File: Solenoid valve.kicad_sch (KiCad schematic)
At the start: 21 parts, among them J2 Conn_01x02, J3 Conn_01x02, J4 Conn_01x02, Q1 S8050, Q2 S8050, U1 BTS443P

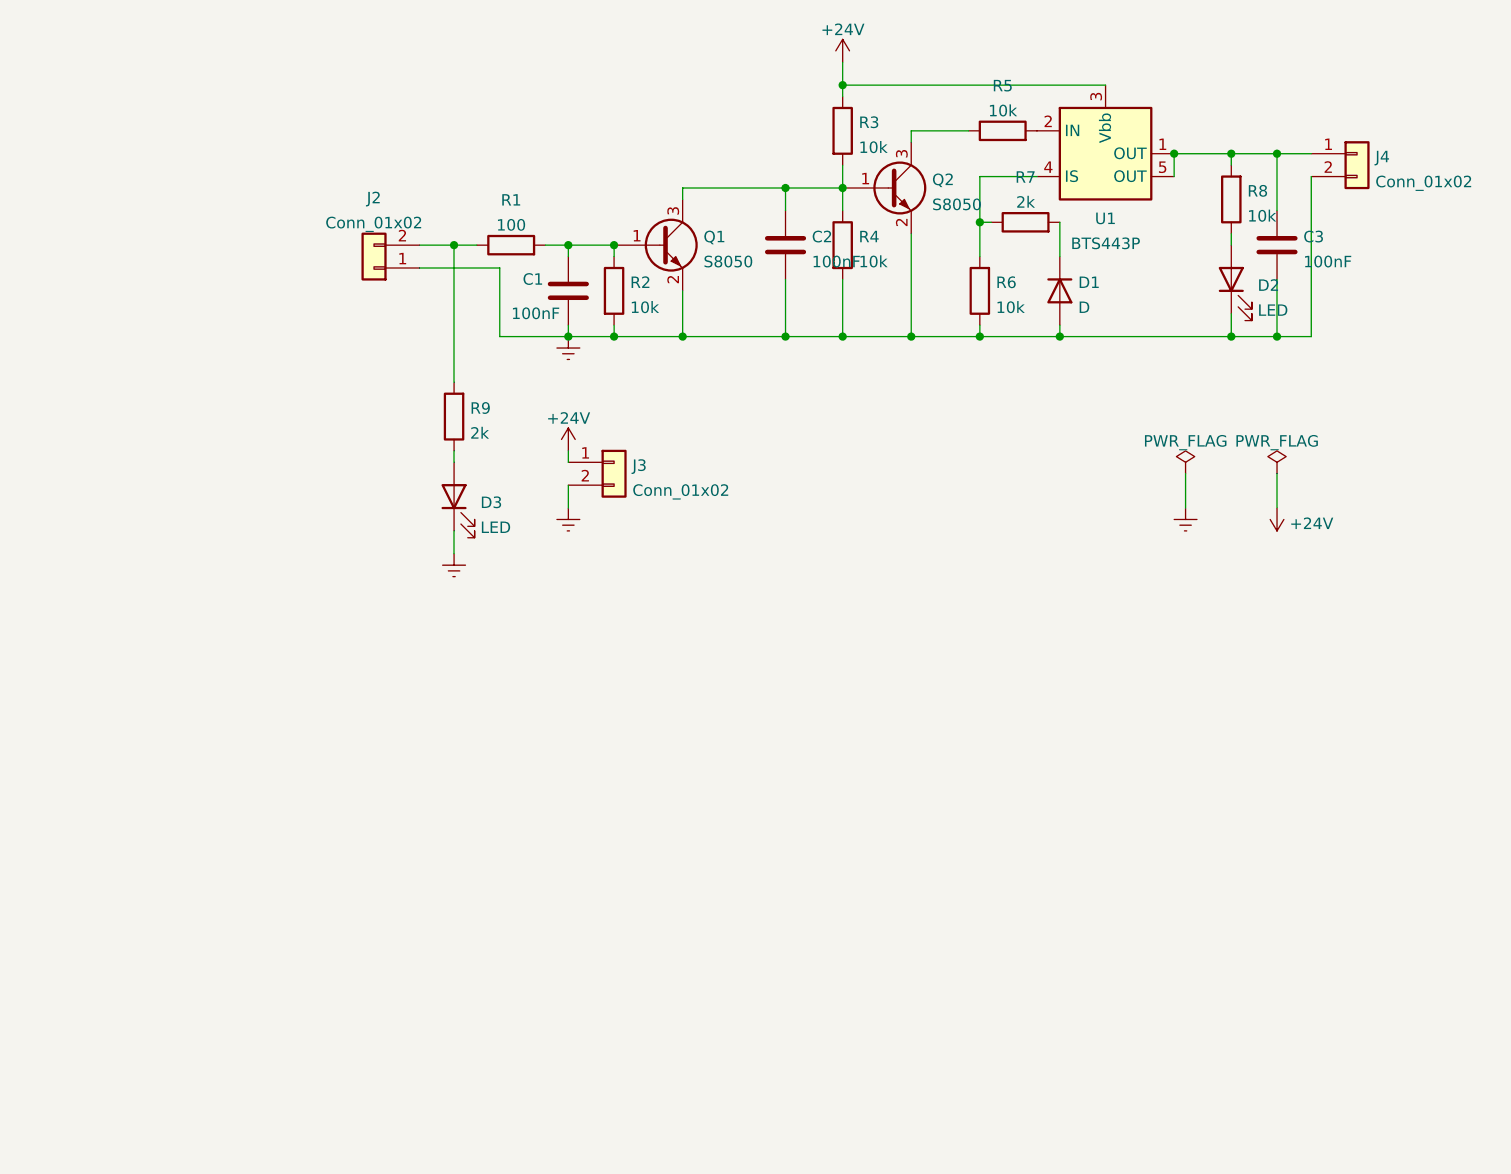
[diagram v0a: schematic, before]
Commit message: Adjustment for full version
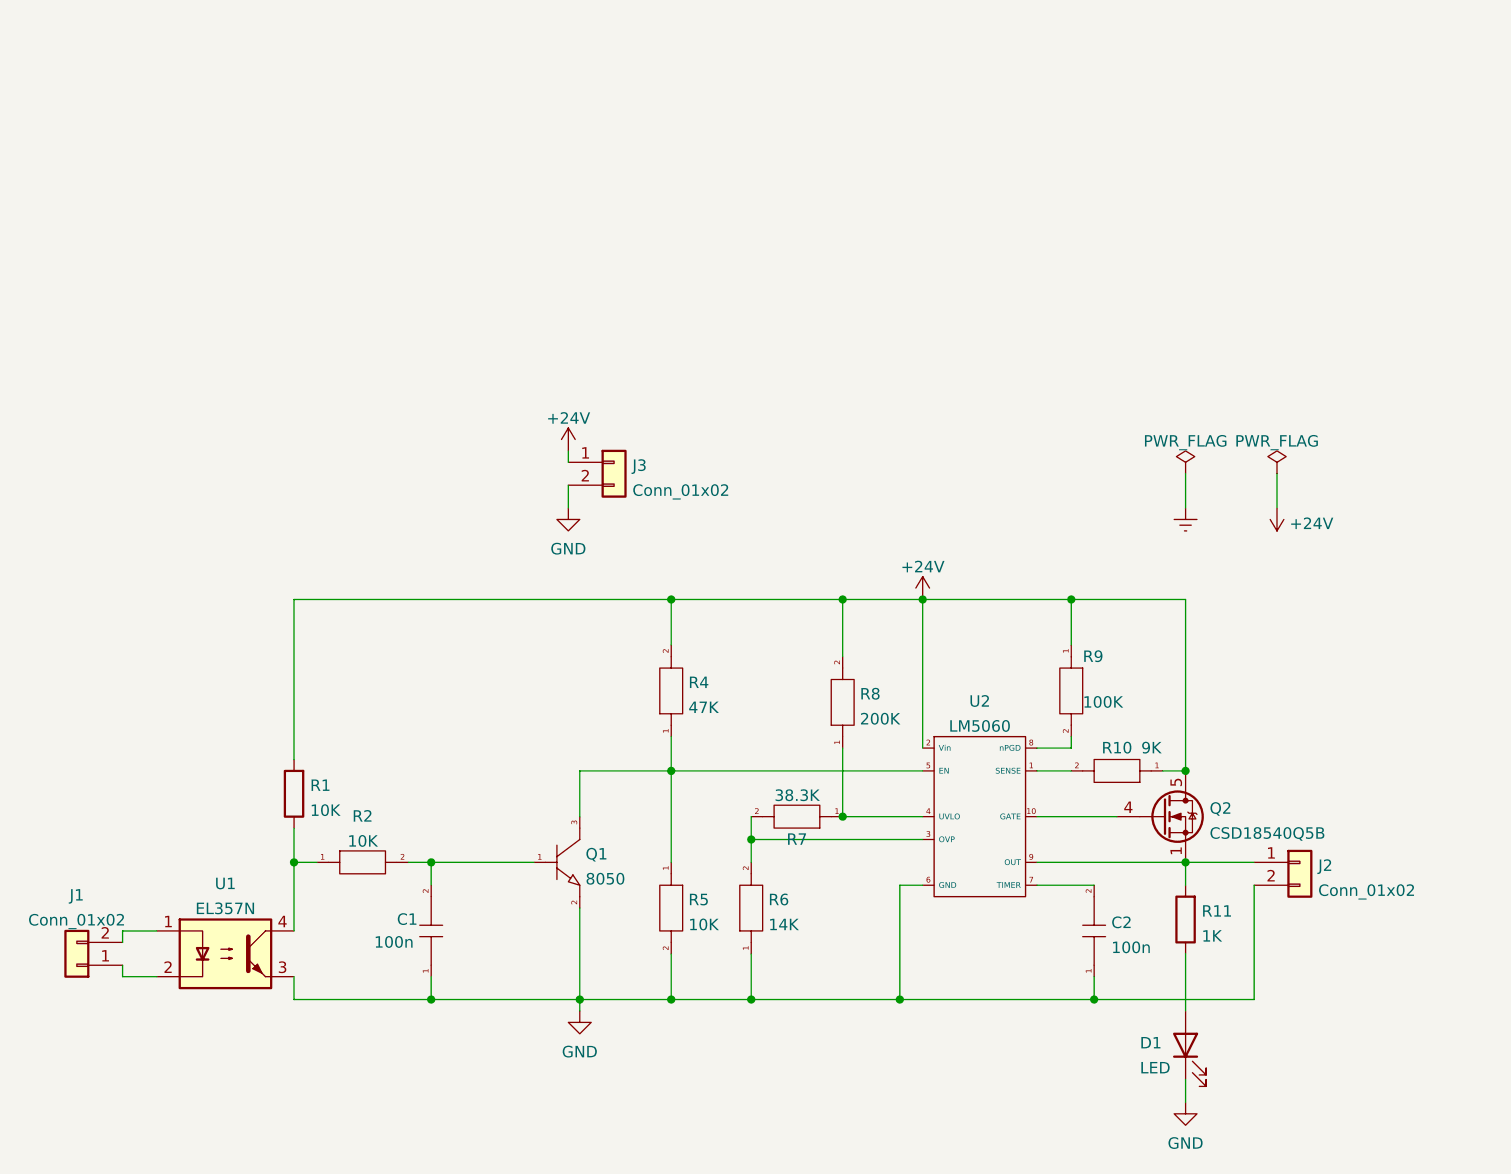
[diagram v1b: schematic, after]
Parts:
- removed C1, C2, C3: 100nF, Capacitor_SMD:C_0603_1608Metric_Pad1.08x0.95mm_HandSolder, symbol Device:C
- removed D1: D, Diode_SMD:D_SOD-123, symbol Device:D
- removed D2, D3: LED, LED_SMD:LED_0603_1608Metric_Pad1.05x0.95mm_HandSolder, symbol Device:LED
- removed J2: Conn_01x02, Connector_JST:JST_GH_SM02B-GHS-TB_1x02-1MP_P1.25mm_Horizontal, symbol Connector_Generic:Conn_01x02
- removed Q1, Q2: S8050, Package_TO_SOT_SMD:SOT-23, symbol Transistor_BJT:S8050
- removed R2, R3, R4, R5, R6, R8: 10k, Resistor_SMD:R_0603_1608Metric_Pad0.98x0.95mm_HandSolder, symbol Device:R
- removed R7, R9: 2k, Resistor_SMD:R_0603_1608Metric_Pad0.98x0.95mm_HandSolder, symbol Device:R
- removed U1: BTS443P, Package_TO_SOT_SMD:TO-252-4, symbol Power_Management:BTS443P
- added C1, C2: 100n, Capacitor_SMD:C_0603_1608Metric, symbol Basic_passive_components:Capacitor
- added D1: LED, Diode_SMD:D_0603_1608Metric, symbol Device:LED
- added J1: Conn_01x02, Connector_JST:JST_GH_SM02B-GHS-TB_1x02-1MP_P1.25mm_Horizontal, symbol Connector_Generic:Conn_01x02
- added Q1: 8050, Package_TO_SOT_SMD:SOT-23, symbol Basic_semiconductor:BJT_NPN
- added Q2: CSD18540Q5B, Package_TO_SOT_SMD:TDSON-8-1, symbol Transistor_FET:CSD18540Q5B
- added R10: 9K, Resistor_SMD:R_0603_1608Metric, symbol Basic_passive_components:Resistor
- added R11: 1K, Resistor_SMD:R_0603_1608Metric, symbol Device:R
- added R2, R5: 10K, Resistor_SMD:R_0603_1608Metric, symbol Basic_passive_components:Resistor
- added R4: 47K, Resistor_SMD:R_0603_1608Metric, symbol Basic_passive_components:Resistor
- added R6: 14K, Resistor_SMD:R_0603_1608Metric, symbol Basic_passive_components:Resistor
- added R7: 38.3K, Resistor_SMD:R_0603_1608Metric, symbol Basic_passive_components:Resistor
- added R8: 200K, Resistor_SMD:R_0603_1608Metric, symbol Basic_passive_components:Resistor
- added R9: 100K, Resistor_SMD:R_0603_1608Metric, symbol Basic_passive_components:Resistor
- added U1: EL357N, Package_SO:SOIC-4_4.55x3.7mm_P2.54mm, symbol Isolator:FODM217C
- added U2: LM5060, Package_SO:VSSOP-10_3x3mm_P0.5mm, symbol Integrated-circuit_transistor_driver:LM5060
- R1: value 100 -> 10K; footprint Resistor_SMD:R_0603_1608Metric_Pad0.98x0.95mm_HandSolder -> Resistor_SMD:R_0603_1608Metric
- renumbered J4 to J2
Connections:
- net +24V: now also R1.2, Q2.5 (D), R10.1, R4.2, R8.2, R9.1, U2.2 (Vin)
- net Earth: no longer J2.2 (Pin_2), J3.2 (Pin_2)
- net at R1.1: now also R2.1, U1.4
- net at J2.1 (Pin_1): now also Q2.1 (S), Q2.2 (S), Q2.3 (S), R11.2, U2.9 (OUT)
- new net: J1.1 (Pin_1), U1.2
- new net: J1.2 (Pin_2), U1.1
- new net: Q2.4 (G), U2.10 (GATE)
- new net: R10.2, U2.1 (SENSE)
- new net: R6.2, R7.2, U2.3 (OVP)
- new net: R7.1, R8.1, U2.4 (UVLO)
- new net: Q1.3 (Collector), R4.1, R5.1, U2.5 (EN)
- new net: C2.2, U2.7 (TIMER)
- new net: R9.2, U2.8 (nPGD)
- new net: D1.2 (A), R11.1
- new net: C1.2, Q1.1 (Base), R2.2
- new net GND: C1.1, C2.1, D1.1 (K), J2.2 (Pin_2), J3.2 (Pin_2), Q1.2 (Emitter), R5.2, R6.1, U1.3, U2.6 (GND)
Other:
- moved on the sheet: J2
